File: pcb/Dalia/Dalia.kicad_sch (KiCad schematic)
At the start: 2 parts

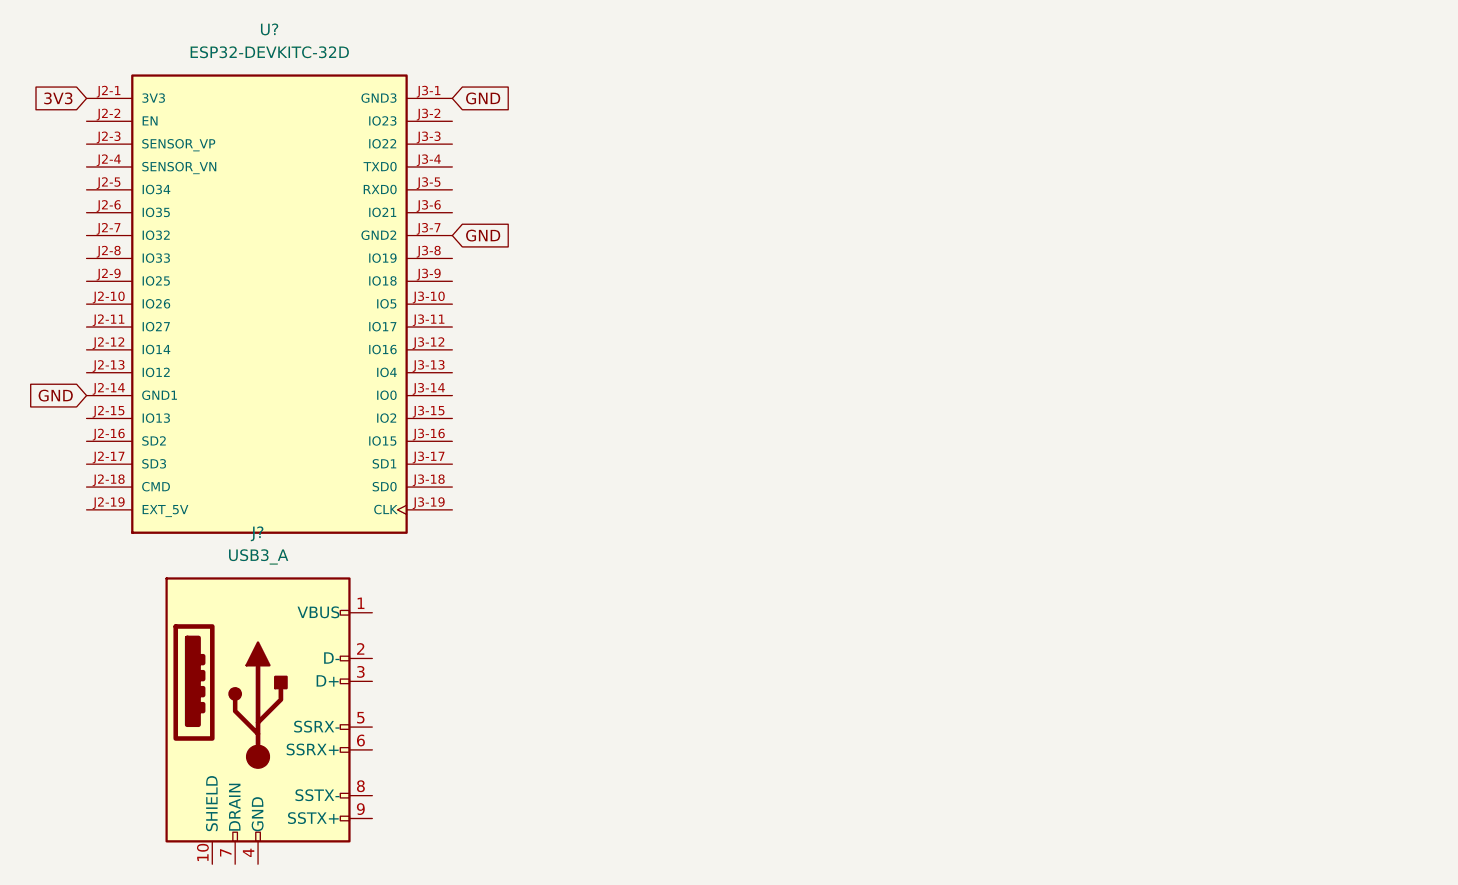
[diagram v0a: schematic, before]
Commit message: Updated PCB
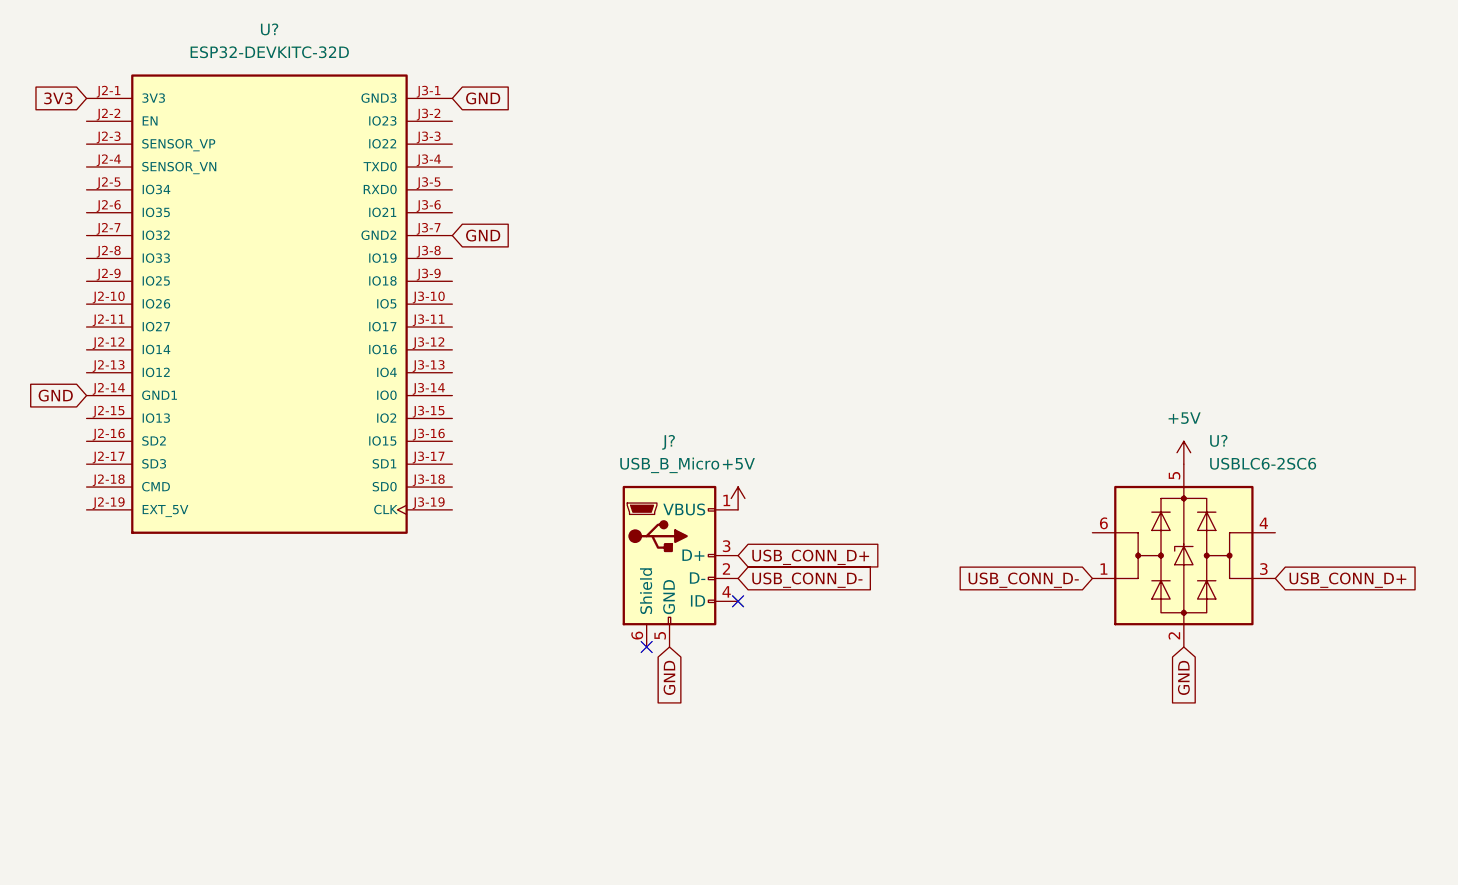
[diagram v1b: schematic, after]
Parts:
- removed J?: USB3_A, symbol Connector:USB3_A
- added J?: USB_B_Micro, symbol Connector:USB_B_Micro
- added U?: USBLC6-2SC6, Package_TO_SOT_SMD:SOT-23-6, symbol Power_Protection:USBLC6-2SC6
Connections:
- net GND: now also J?.5 (GND), U?.2 (GND)
- new net +5V: J?.1 (VBUS), U?.5 (VBUS)
- new net USB_CONN_D+: J?.3 (D+), U?.3 (I/O2)
- new net USB_CONN_D-: J?.2 (D-), U?.1 (I/O1)
- no-connect marks 0 -> 2
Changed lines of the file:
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@@
     (company "AndromedaHelix")
   )
+  (no_connect (at 190.5 130.81))
+  (no_connect (at 200.66 125.73))
+  (global_label "GND" (shape input) (at 193.04 130.81 270) (fields_autoplaced)
+    (effects (font (size 1.27 1.27)) (justify right))
+    (property "Intersheet References" "${INTERSHEET_REFS}" (id 0) (at 192.9606 137.0936 90)
+      (effects (font (size 1.27 1.27)) (justify right) hide)
+    )
+  )
   (global_label "GND" (shape input) (at 168.91 69.85 0) (fields_autoplaced)
     (effects (font (size 1.27 1.27)) (justify left))
@@
     )
   )
+  (global_label "USB_CONN_D-" (shape input) (at 200.66 123.19 0) (fields_autoplaced)
+    (effects (font (size 1.27 1.27)) (justify left))
+    (property "Intersheet References" "${INTERSHEET_REFS}" (id 0) (at 216.9221 123.1106 0)
+      (effects (font (size 1.27 1.27)) (justify left) hide)
+    )
+  )
   (global_label "GND" (shape input) (at 168.91 85.09 0) (fields_autoplaced)
     (effects (font (size 1.27 1.27)) (justify left))
@@
     )
   )
+  (global_label "USB_CONN_D-" (shape input) (at 240.03 123.19 180) (fields_autoplaced)
+    (effects (font (size 1.27 1.27)) (justify right))
+    (property "Intersheet References" "${INTERSHEET_REFS}" (id 0) (at 223.7679 123.2694 0)
+      (effects (font (size 1.27 1.27)) (justify right) hide)
+    )
+  )
   (global_label "GND" (shape input) (at 128.27 102.87 180) (fields_autoplaced)
     (effects (font (size 1.27 1.27)) (justify right))
@@
       (effects (font (size 1.27 1.27)) (justify right) hide)
     )
+  )
+  (global_label "GND" (shape input) (at 250.19 130.81 270) (fields_autoplaced)
+    (effects (font (size 1.27 1.27)) (justify right))
+    (property "Intersheet References" "${INTERSHEET_REFS}" (id 0) (at 250.1106 137.0936 90)
+      (effects (font (size 1.27 1.27)) (justify right) hide)
+    )
+  )
+  (global_label "USB_CONN_D+" (shape input) (at 260.35 123.19 0) (fields_autoplaced)
+    (effects (font (size 1.27 1.27)) (justify left))
+    (property "Intersheet References" "${INTERSHEET_REFS}" (id 0) (at 276.6121 123.1106 0)
+      (effects (font (size 1.27 1.27)) (justify left) hide)
+    )
+  )
+  (global_label "USB_CONN_D+" (shape input) (at 200.66 120.65 0) (fields_autoplaced)
+    (effects (font (size 1.27 1.27)) (justify left))
+    (property "Intersheet References" "${INTERSHEET_REFS}" (id 0) (at 216.9221 120.5706 0)
+      (effects (font (size 1.27 1.27)) (justify left) hide)
+    )
+  )
+  (symbol (lib_id "Power_Protection:USBLC6-2SC6") (at 250.19 120.65 0) (unit 1)
+    (in_bom yes) (on_board yes) (fields_autoplaced)
+    (property "Reference" "U?" (id 0) (at 252.9587 107.95 0)
+      (effects (font (size 1.27 1.27)) (justify left))
+    )
+    (property "Value" "USBLC6-2SC6" (id 1) (at 252.9587 110.49 0)
+      (effects (font (size 1.27 1.27)) (justify left))
+    )
+    (property "Footprint" "Package_TO_SOT_SMD:SOT-23-6" (id 2) (at 250.19 133.35 0)
+      (effects (font (size 1.27 1.27)) hide)
+    )
+    (property "Datasheet" "https://www.st.com/resource/en/datasheet/usblc6-2.pdf" (id 3) (at 255.27 111.76 0)
+      (effects (font (size 1.27 1.27)) hide)
+    )
+    (pin "1")
+    (pin "2")
+    (pin "3")
+    (pin "4")
+    (pin "5")
+    (pin "6")
   )
   (symbol (lib_id "ESP32-DEVKITC-32D:ESP32-DEVKITC-32D") (at 148.59 92.71 0) (unit 1)
@@
     (pin "J3-9")
   )
-  (symbol (lib_id "Connector:USB3_A") (at 147.32 137.16 0) (unit 1)
-    (in_bom yes) (on_board yes) (fields_autoplaced)
-    (property "Reference" "J?" (id 0) (at 147.32 118.11 0))
-    (property "Value" "USB3_A" (id 1) (at 147.32 120.65 0))
-    (property "Footprint" "" (id 2) (at 151.13 134.62 0)
-      (effects (font (size 1.27 1.27)) hide)
-    )
-    (property "Datasheet" "~" (id 3) (at 151.13 134.62 0)
-      (effects (font (size 1.27 1.27)) hide)
-    )
-    (pin "1")
-    (pin "10")
+  (symbol (lib_id "Connector:USB_B_Micro") (at 193.04 120.65 0) (unit 1)
+    (in_bom yes) (on_board yes) (fields_autoplaced)
+    (property "Reference" "J?" (id 0) (at 193.04 107.95 0))
+    (property "Value" "USB_B_Micro" (id 1) (at 193.04 110.49 0))
+    (property "Footprint" "" (id 2) (at 196.85 121.92 0)
+      (effects (font (size 1.27 1.27)) hide)
+    )
+    (property "Datasheet" "~" (id 3) (at 196.85 121.92 0)
+      (effects (font (size 1.27 1.27)) hide)
+    )
+    (pin "1")
     (pin "2")
     (pin "3")
@@
     (pin "5")
     (pin "6")
-    (pin "7")
-    (pin "8")
-    (pin "9")
+  )
+  (symbol (lib_id "power:+5V") (at 200.66 115.57 0) (unit 1)
+    (in_bom yes) (on_board yes) (fields_autoplaced)
+    (property "Reference" "#PWR?" (id 0) (at 200.66 119.38 0)
+      (effects (font (size 1.27 1.27)) hide)
+    )
+    (property "Value" "+5V" (id 1) (at 200.66 110.49 0))
+    (property "Footprint" "" (id 2) (at 200.66 115.57 0)
+      (effects (font (size 1.27 1.27)) hide)
+    )
+    (property "Datasheet" "" (id 3) (at 200.66 115.57 0)
+      (effects (font (size 1.27 1.27)) hide)
+    )
+    (pin "1")
+  )
+  (symbol (lib_id "power:+5V") (at 250.19 110.49 0) (unit 1)
+    (in_bom yes) (on_board yes) (fields_autoplaced)
+    (property "Reference" "#PWR?" (id 0) (at 250.19 114.3 0)
+      (effects (font (size 1.27 1.27)) hide)
+    )
+    (property "Value" "+5V" (id 1) (at 250.19 105.41 0))
+    (property "Footprint" "" (id 2) (at 250.19 110.49 0)
+      (effects (font (size 1.27 1.27)) hide)
+    )
+    (property "Datasheet" "" (id 3) (at 250.19 110.49 0)
+      (effects (font (size 1.27 1.27)) hide)
+    )
+    (pin "1")
   )
   (sheet_instances
@@
   )
   (symbol_instances
-    (path "/8f4e2a89-f072-458e-afb3-673b3d29090b"
-      (reference "J?") (unit 1) (value "USB3_A") (footprint "")
+    (path "/acbc059b-c5dd-4e78-9076-4d0d5dff753c"
+      (reference "#PWR?") (unit 1) (value "+5V") (footprint "")
+    )
+    (path "/f56ce442-d11b-40b3-8c54-dce5c48e1dbe"
+      (reference "#PWR?") (unit 1) (value "+5V") (footprint "")
+    )
+    (path "/78f58473-7315-4827-b173-aa781c6fb7e3"
+      (reference "J?") (unit 1) (value "USB_B_Micro") (footprint "")
+    )
+    (path "/38a38a2f-3588-41e0-966c-b7cba737b687"
+      (reference "U?") (unit 1) (value "USBLC6-2SC6") (footprint "Package_TO_SOT_SMD:SOT-23-6")
     )
     (path "/41af8376-181e-4c15-96fd-62e389a090fe"
